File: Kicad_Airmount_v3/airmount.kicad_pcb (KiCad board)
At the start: 2 copper layers, 24.1 x 28.1 mm, 4 parts, among them J1 JST, M1 Motor_DC, M2 Motor_DC

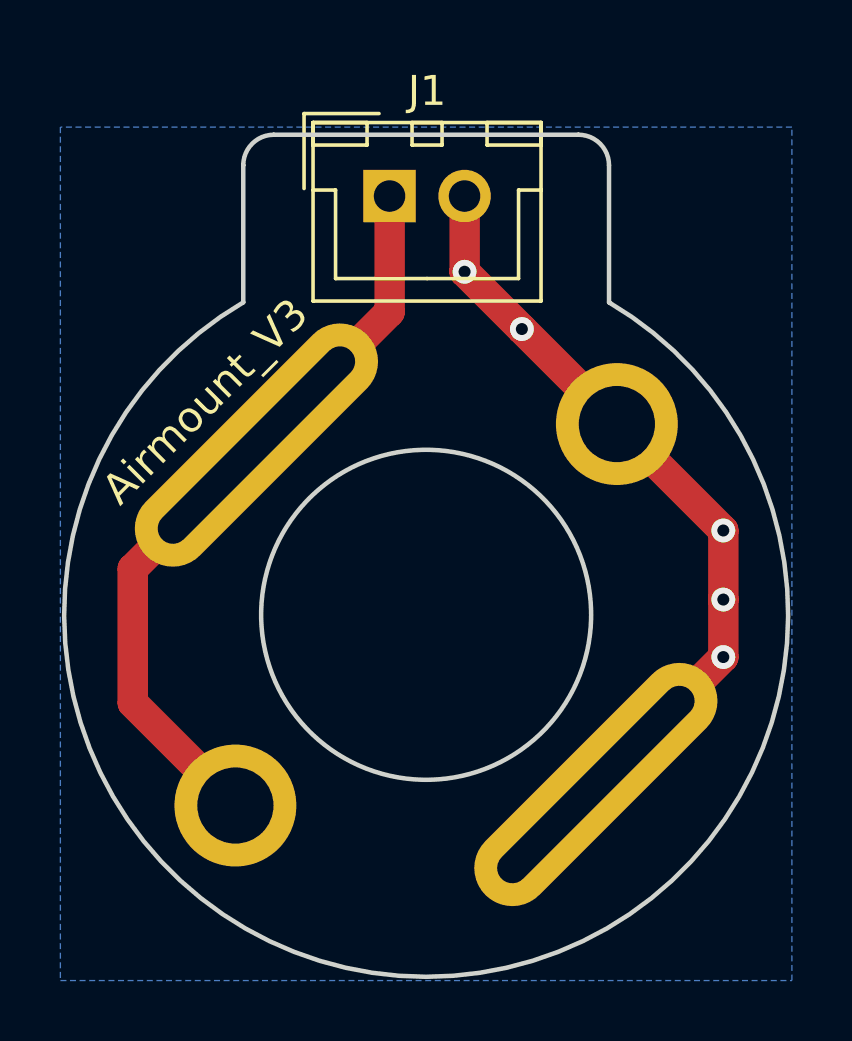
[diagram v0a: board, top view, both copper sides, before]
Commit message: Airmount _v2 and _v3 revised gerbers
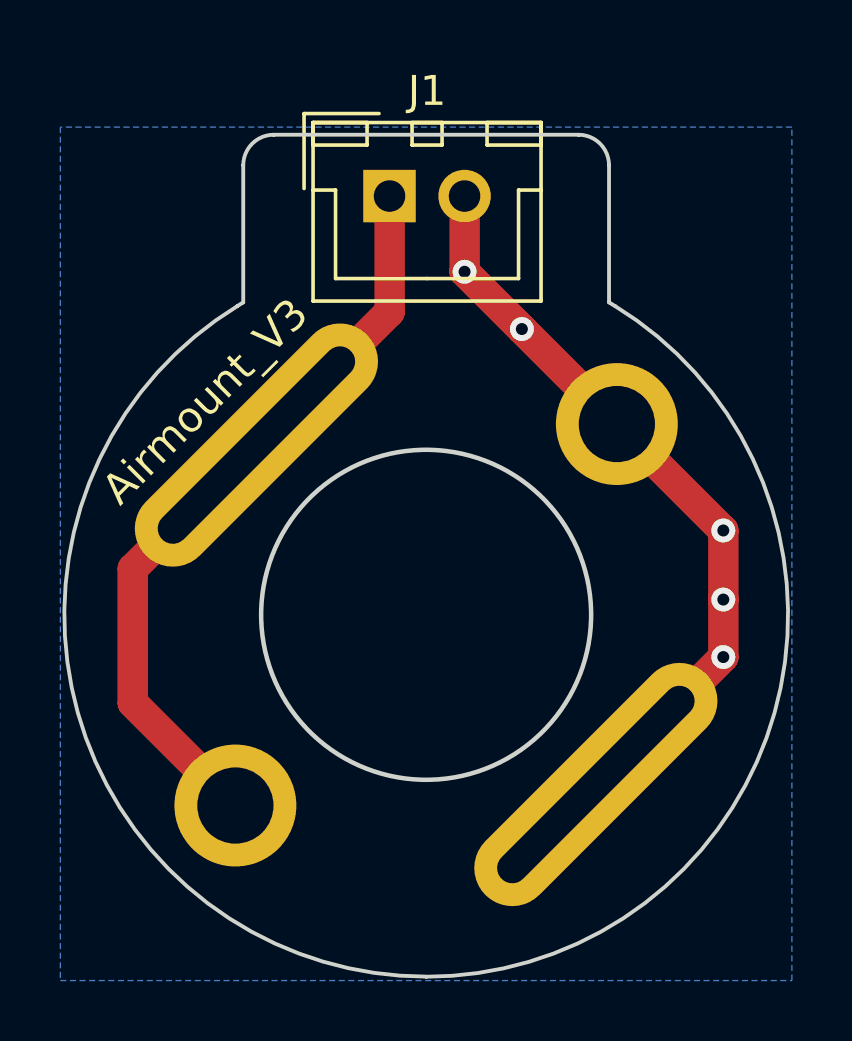
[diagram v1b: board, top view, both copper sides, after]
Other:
- outline, holes or cut-outs redrawn
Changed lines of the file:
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@@
   (general
     (thickness 1.6)
-    (drawings 11)
+    (drawings 14)
     (tracks 20)
     (zones 0)
@@
     (0 F.Cu signal)
     (31 B.Cu signal)
-    (32 B.Adhes user hide)
-    (33 F.Adhes user hide)
-    (34 B.Paste user hide)
-    (35 F.Paste user hide)
+    (32 B.Adhes user)
+    (33 F.Adhes user)
+    (34 B.Paste user)
+    (35 F.Paste user)
     (36 B.SilkS user)
     (37 F.SilkS user)
-    (38 B.Mask user hide)
-    (39 F.Mask user hide)
-    (40 Dwgs.User user hide)
-    (41 Cmts.User user hide)
-    (42 Eco1.User user hide)
-    (43 Eco2.User user hide)
+    (38 B.Mask user)
+    (39 F.Mask user)
+    (40 Dwgs.User user)
+    (41 Cmts.User user)
+    (42 Eco1.User user)
+    (43 Eco2.User user)
     (44 Edge.Cuts user)
-    (45 Margin user hide)
-    (46 B.CrtYd user hide)
-    (47 F.CrtYd user hide)
+    (45 Margin user)
+    (46 B.CrtYd user)
+    (47 F.CrtYd user)
     (48 B.Fab user hide)
     (49 F.Fab user hide)
@@
     (uvia_min_size 0.2)
     (uvia_min_drill 0.1)
-    (edge_width 0.15)
-    (segment_width 0.2)
-    (pcb_text_width 0.3)
-    (pcb_text_size 1.5 1.5)
-    (mod_edge_width 0.15)
-    (mod_text_size 1 1)
-    (mod_text_width 0.15)
+    (edge_width 0.127)
+    (segment_width 0.2032)
+    (pcb_text_width 0.254)
+    (pcb_text_size 1.524 1.016)
+    (mod_edge_width 0.127)
+    (mod_text_size 1.016 1.016)
+    (mod_text_width 0.127)
     (pad_size 4 4)
     (pad_drill 2.5)
@@
       (creategerberjobfile false)
       (excludeedgelayer true)
-      (linewidth 0.100000)
+      (linewidth 0.127000)
       (plotframeref false)
       (viasonmask false)
@@
     )
   )
+  (gr_arc (start 127 88.9) (end 120.70334 78.613) (angle -148.529251) (layer Edge.Cuts) (width 0.127))
+  (gr_arc (start 127 88.9) (end 127 100.965) (angle -148.5189608) (layer Edge.Cuts) (width 0.127))
+  (gr_line (start 133.2992 78.61046) (end 133.096 78.486) (layer Edge.Cuts) (width 0.127))
+  (gr_line (start 120.7008 78.613) (end 120.904 78.486) (layer Edge.Cuts) (width 0.127))
   (gr_text Airmount_V3 (at 119.634 81.915 45) (layer B.SilkS)
     (effects (font (size 1.016 1.016) (thickness 0.1524)) (justify mirror))
@@
     (arrow2b (pts (xy 114.935 102.87) (xy 116.061504 102.283579)))
   )
-  (gr_arc (start 132.08 73.914) (end 133.096 73.914) (angle -90) (layer Edge.Cuts) (width 0.15))
-  (gr_arc (start 121.92 73.914) (end 121.92 72.898) (angle -90) (layer Edge.Cuts) (width 0.15))
-  (gr_line (start 120.904 73.914) (end 120.904 78.486) (layer Edge.Cuts) (width 0.15))
-  (gr_line (start 132.08 72.898) (end 121.92 72.898) (layer Edge.Cuts) (width 0.15))
-  (gr_line (start 133.096 78.486) (end 133.096 73.914) (layer Edge.Cuts) (width 0.15))
+  (gr_arc (start 132.08 73.914) (end 133.096 73.914) (angle -90) (layer Edge.Cuts) (width 0.127))
+  (gr_arc (start 121.92 73.914) (end 121.92 72.898) (angle -90) (layer Edge.Cuts) (width 0.127))
+  (gr_line (start 120.904 73.914) (end 120.904 78.486) (layer Edge.Cuts) (width 0.127))
+  (gr_line (start 132.08 72.898) (end 121.92 72.898) (layer Edge.Cuts) (width 0.127))
+  (gr_line (start 133.096 78.486) (end 133.096 73.914) (layer Edge.Cuts) (width 0.127))
   (gr_circle (center 127 88.9) (end 132.5 88.9) (layer Edge.Cuts) (width 0.15))
-  (gr_arc (start 127 88.9) (end 120.904 78.486) (angle -299.3135022) (layer Edge.Cuts) (width 0.15))
   (segment (start 128.2808 77.464758) (end 128.2808 77.464758) (width 1.016) (layer F.Cu) (net 1))
   (segment (start 128.2808 74.9418) (end 128.2808 77.464758) (width 1.016) (layer F.Cu) (net 1))
